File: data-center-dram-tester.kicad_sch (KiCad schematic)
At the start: 7 parts, among them M1 1296.2013

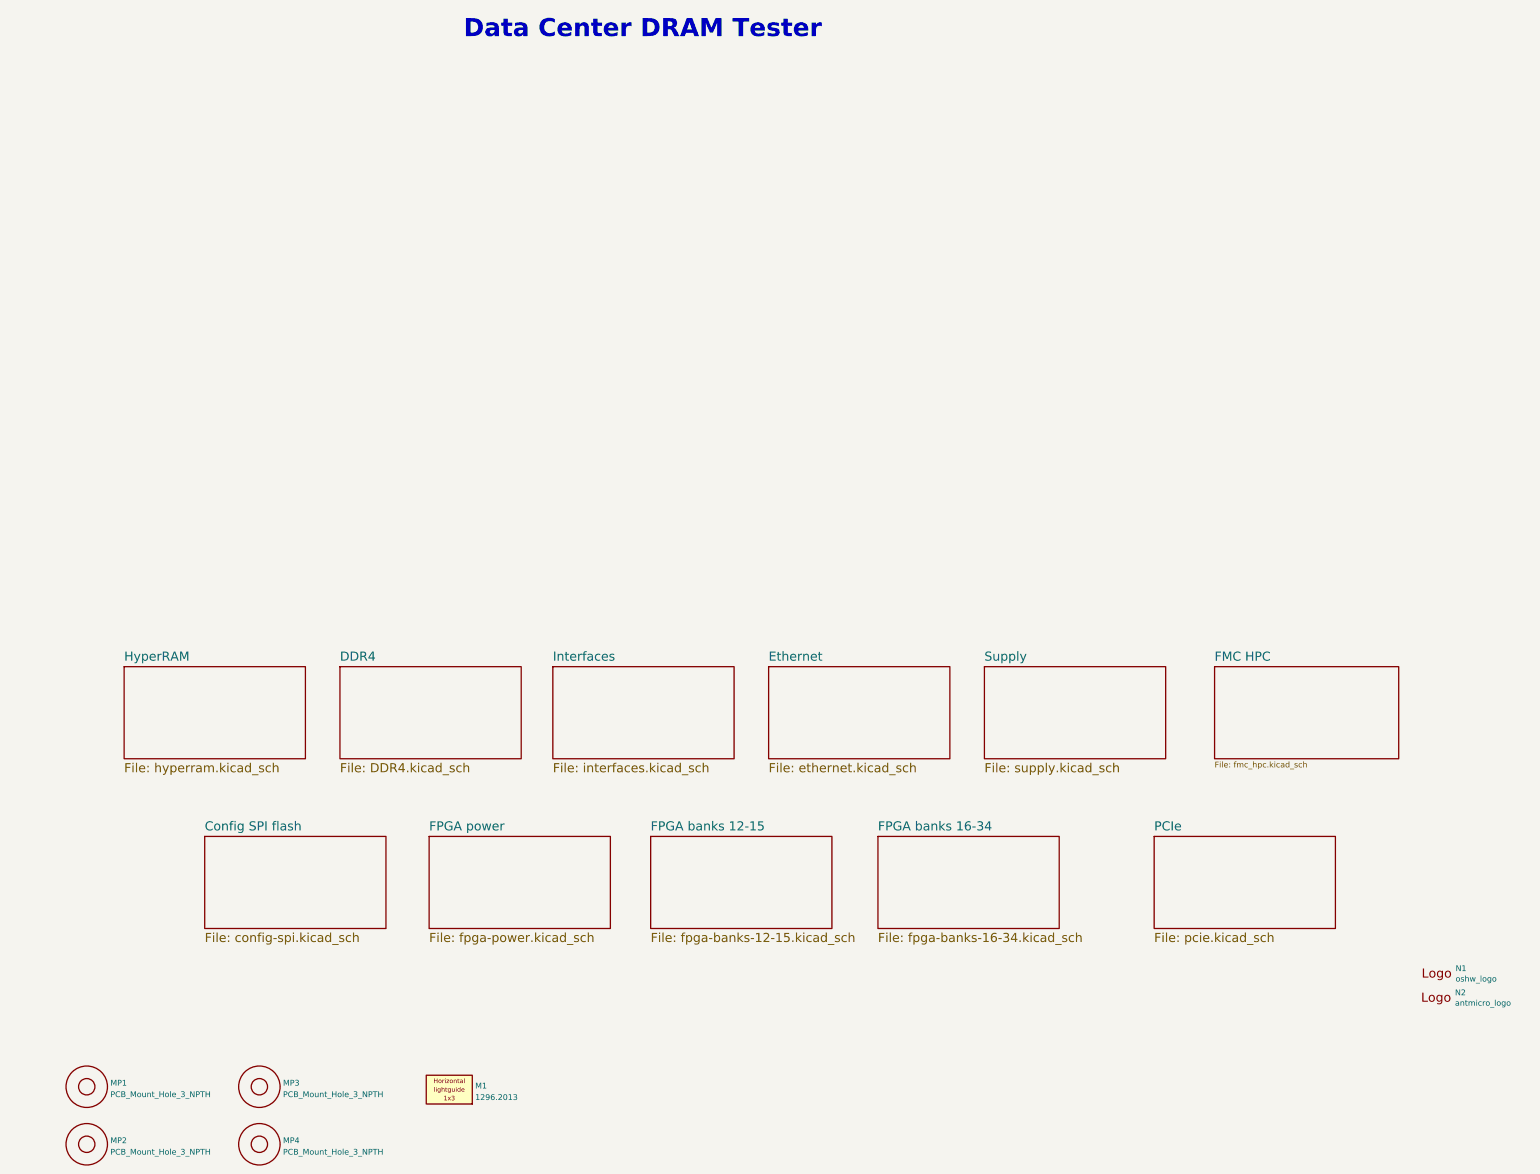
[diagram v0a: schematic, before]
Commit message: Cleanup schematic
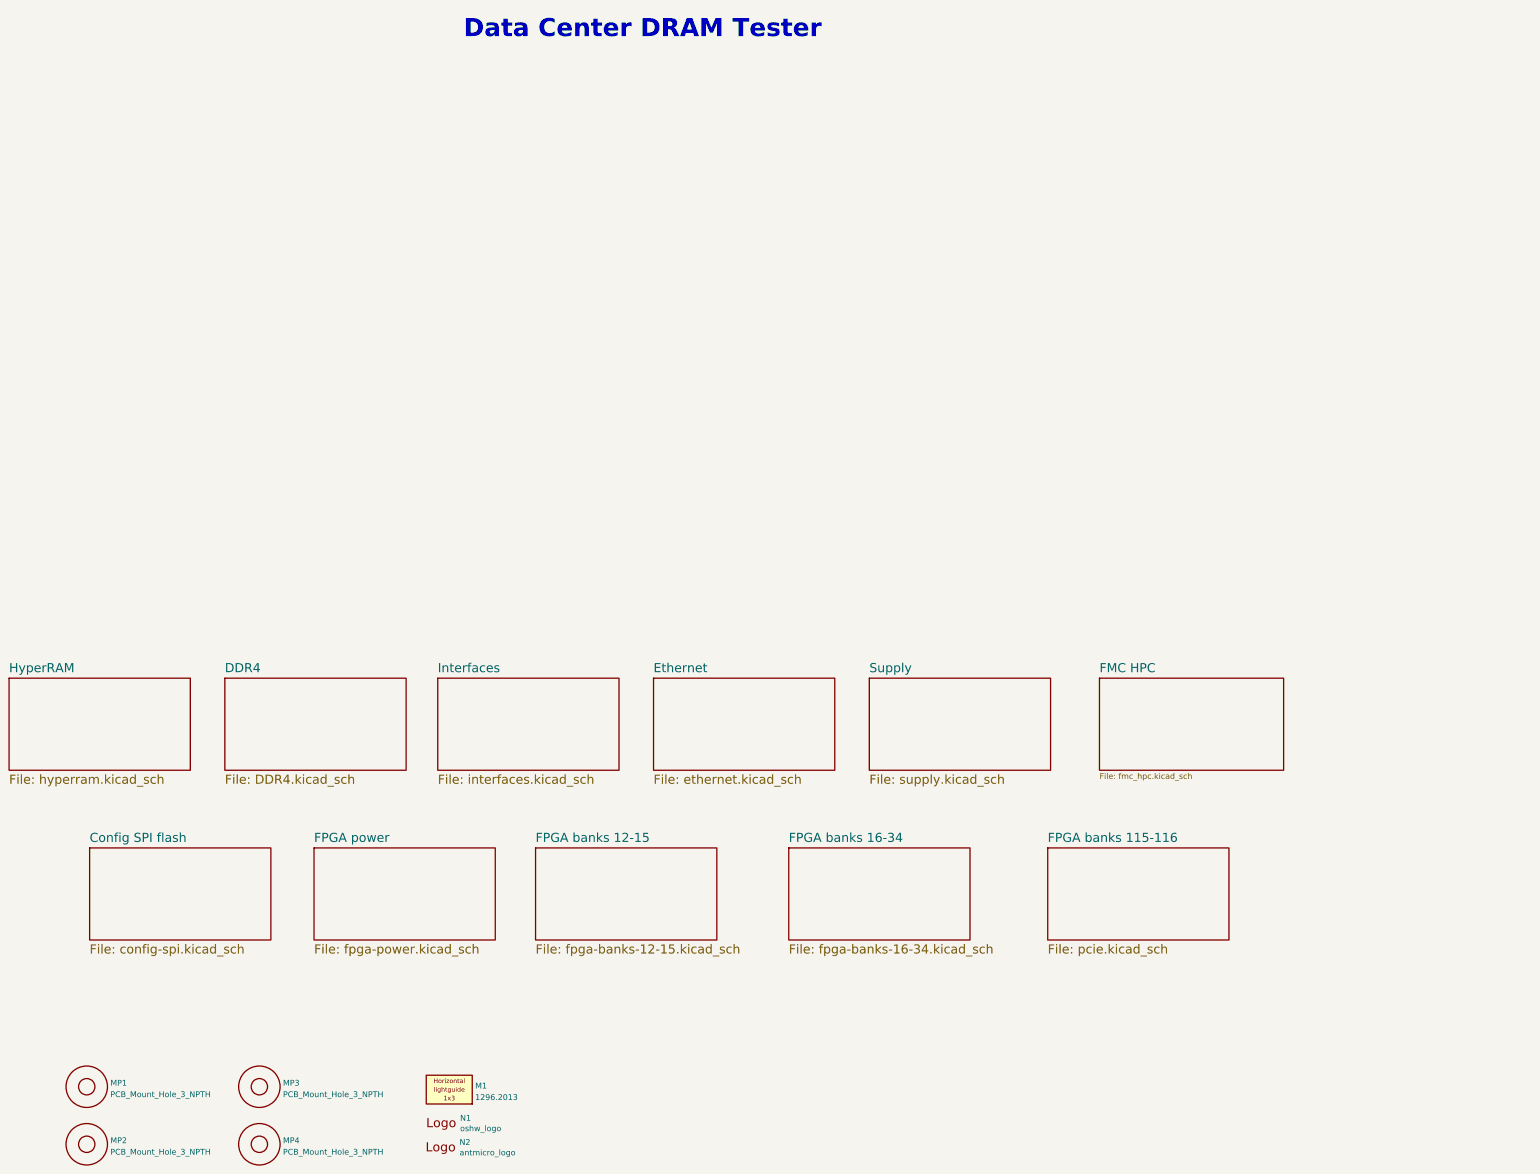
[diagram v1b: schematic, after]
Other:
- sheet PCIe renamed FPGA banks 115-116
- moved on the sheet: N1, N2
